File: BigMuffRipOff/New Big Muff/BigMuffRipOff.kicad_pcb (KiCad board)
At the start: 4 copper layers, 59.3 x 32 mm, 70 parts, among them J1 Conn_02x08_Odd_Even, Q1 BC549, Q2 BC549, Q3 BC549, Q4 BC549, U1 TPL0501-100DCNR, U10 LM2940IMP-9.0/NOPB, U2 TPL0501-100DCNR, U3 TPL0501-100DCNR, U4 TL071HIDBVR, U5 TL071HIDBVR, U6 ADP7118AUJZ-4.5-R7, U7 TL071HIDBVR, U8 TPL0501-100DCNR

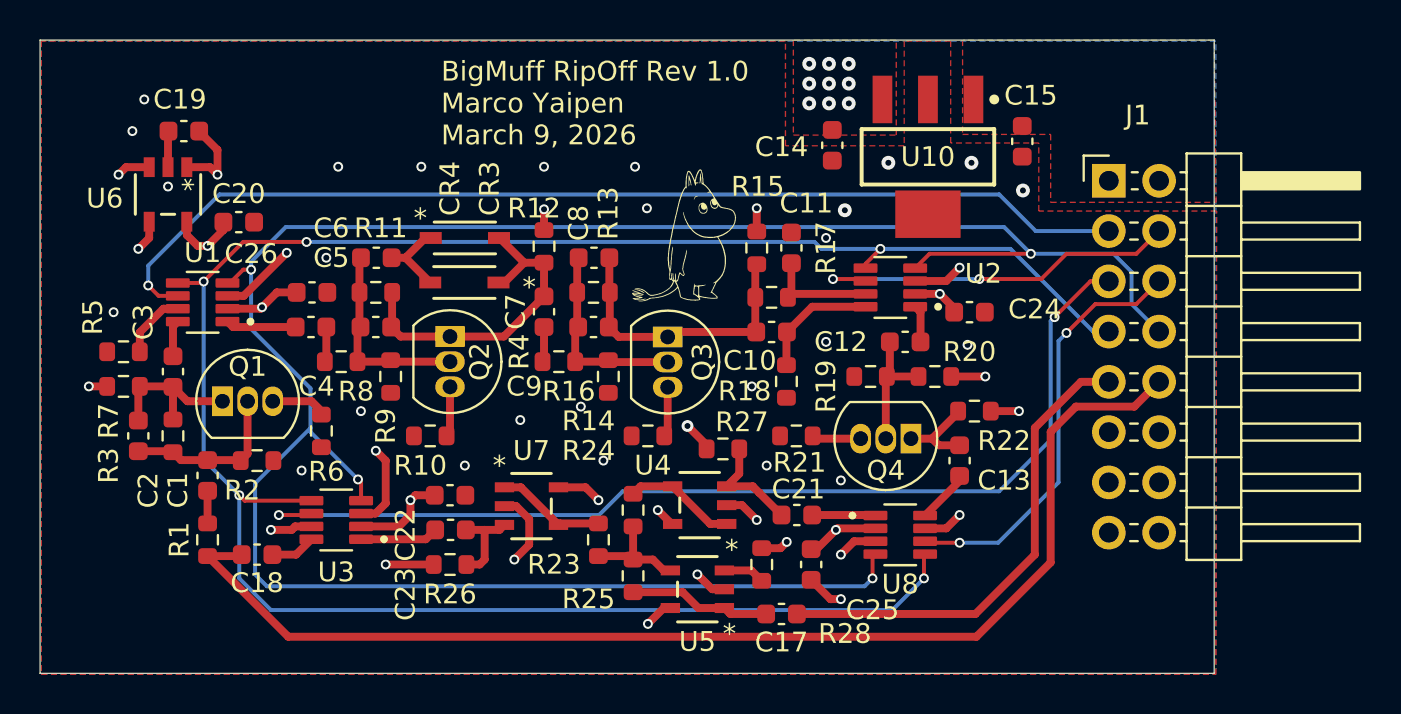
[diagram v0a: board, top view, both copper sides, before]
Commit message: big muff connector fixed i think?
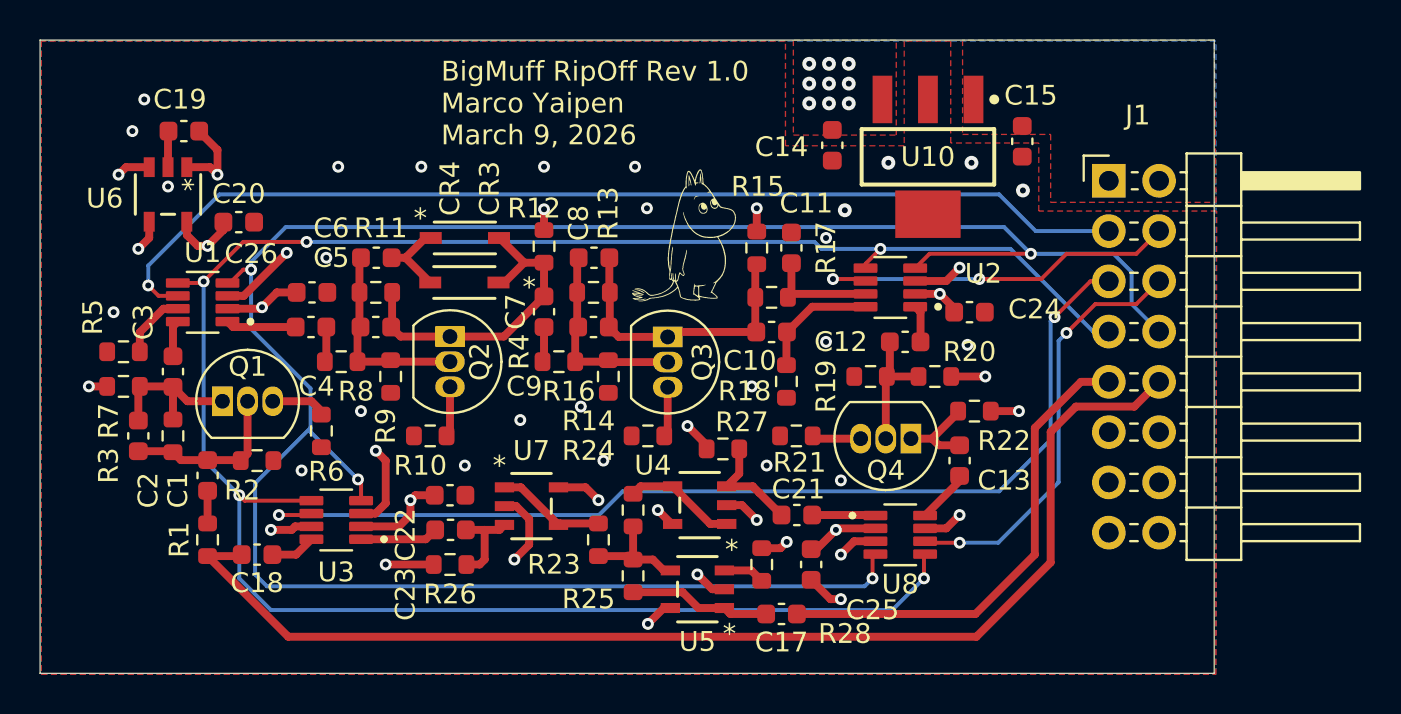
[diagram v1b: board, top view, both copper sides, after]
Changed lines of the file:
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@@
 	(via
 		(at 135.2 95.75)
-		(size 0.5)
+		(size 0.6)
 		(drill 0.3)
 		(layers "F.Cu" "B.Cu")
@@
 	(via
 		(at 152 92.25)
-		(size 0.5)
+		(size 0.6)
 		(drill 0.3)
 		(layers "F.Cu" "B.Cu")
@@
 	(via
 		(at 128.2 75.6)
-		(size 0.5)
+		(size 0.6)
 		(drill 0.3)
 		(layers "F.Cu" "B.Cu")
@@
 	(via
 		(at 160.25 92.5)
-		(size 0.5)
+		(size 0.6)
 		(drill 0.3)
 		(layers "F.Cu" "B.Cu")
@@
 	(via
 		(at 127.25 84.75)
-		(size 0.5)
+		(size 0.6)
 		(drill 0.3)
 		(layers "F.Cu" "B.Cu")
@@
 	(via
 		(at 163.25 86.25)
-		(size 0.5)
+		(size 0.6)
 		(drill 0.3)
 		(layers "F.Cu" "B.Cu")
@@
 	(via
 		(at 145 92.5)
-		(size 0.5)
+		(size 0.6)
 		(drill 0.3)
 		(layers "F.Cu" "B.Cu")
@@
 	(via
 		(at 159.75 95.25)
-		(size 0.5)
+		(size 0.6)
 		(drill 0.3)
 		(layers "F.Cu" "B.Cu")
@@
 	(via
 		(at 138 82)
-		(size 0.5)
+		(size 0.6)
 		(drill 0.3)
 		(layers "F.Cu" "B.Cu")
@@
 	(via
 		(at 136.75 92.75)
-		(size 0.5)
+		(size 0.6)
 		(drill 0.3)
 		(layers "F.Cu" "B.Cu")
@@
 	(via
 		(at 163.25 81)
-		(size 0.5)
+		(size 0.6)
 		(drill 0.3)
 		(layers "F.Cu" "B.Cu")
@@
 	(via
 		(at 154.2 79.5)
-		(size 0.5)
+		(size 0.6)
 		(drill 0.3)
 		(layers "F.Cu" "B.Cu")
@@
 	(via
 		(at 153.6 77.4)
-		(size 0.5)
+		(size 0.6)
 		(drill 0.3)
 		(layers "F.Cu" "B.Cu")
@@
 	(via
 		(at 142.8 77.4)
-		(size 0.5)
+		(size 0.6)
 		(drill 0.3)
 		(layers "F.Cu" "B.Cu")
@@
 	(via
 		(at 170 82.5)
-		(size 0.5)
+		(size 0.6)
 		(drill 0.3)
 		(layers "F.Cu" "B.Cu")
@@
 	(via
 		(at 149 77.4)
-		(size 0.5)
+		(size 0.6)
 		(drill 0.3)
 		(layers "F.Cu" "B.Cu")
@@
 	(via
 		(at 164 99.25)
-		(size 0.5)
+		(size 0.6)
 		(drill 0.3)
 		(layers "F.Cu" "B.Cu")
@@
 	(via
 		(at 164 97)
-		(size 0.5)
+		(size 0.6)
 		(drill 0.3)
 		(layers "F.Cu" "B.Cu")
@@
 	(via
 		(at 170 95)
-		(size 0.5)
+		(size 0.6)
 		(drill 0.3)
 		(layers "F.Cu" "B.Cu")
@@
 	(via
 		(at 147.8 90.2)
-		(size 0.5)
+		(size 0.6)
 		(drill 0.3)
 		(layers "F.Cu" "B.Cu")
@@
 	(via
 		(at 130 78.4)
-		(size 0.5)
+		(size 0.6)
 		(drill 0.3)
 		(layers "F.Cu" "B.Cu")
@@
 	(via
 		(at 139.75 89.75)
-		(size 0.5)
+		(size 0.6)
 		(drill 0.3)
 		(layers "F.Cu" "B.Cu")
@@
 	(via
 		(at 140.5 91.75)
-		(size 0.5)
+		(size 0.6)
 		(drill 0.3)
 		(layers "F.Cu" "B.Cu")
@@
 	(via
 		(at 156.75 98)
-		(size 0.5)
+		(size 0.6)
 		(drill 0.3)
 		(layers "F.Cu" "B.Cu")
@@
 	(via
 		(at 136 81.75)
-		(size 0.5)
+		(size 0.6)
 		(drill 0.3)
 		(layers "F.Cu" "B.Cu")
@@
 	(via
 		(at 147.5 97.25)
-		(size 0.5)
+		(size 0.6)
 		(drill 0.3)
 		(layers "F.Cu" "B.Cu")
@@
 	(via
 		(at 170.4 86.4)
-		(size 0.5)
+		(size 0.6)
 		(drill 0.3)
 		(layers "F.Cu" "B.Cu")
@@
 	(via
 		(at 150.860363 89.520726)
-		(size 0.5)
+		(size 0.6)
 		(drill 0.3)
 		(layers "F.Cu" "B.Cu")
@@
 	(via
 		(at 164 93.25)
-		(size 0.5)
+		(size 0.6)
 		(drill 0.3)
 		(layers "F.Cu" "B.Cu")
@@
 	(via
 		(at 128.8 74)
-		(size 0.5)
+		(size 0.6)
 		(drill 0.3)
 		(layers "F.Cu" "B.Cu")
@@
 	(via
 		(at 138.6 77.4)
-		(size 0.5)
+		(size 0.6)
 		(drill 0.3)
 		(layers "F.Cu" "B.Cu")
@@
 	(via
 		(at 159.5 88.5)
-		(size 0.5)
+		(size 0.6)
 		(drill 0.3)
 		(layers "F.Cu" "B.Cu")
@@
 	(via
 		(at 127.5 77.8)
-		(size 0.5)
+		(size 0.6)
 		(drill 0.3)
 		(layers "F.Cu" "B.Cu")
@@
 	(via
 		(at 132.5 77.8)
-		(size 0.5)
+		(size 0.6)
 		(drill 0.3)
 		(layers "F.Cu" "B.Cu")
@@
 	(via
 		(at 154.25 100.5)
-		(size 0.5)
+		(size 0.6)
 		(drill 0.3)
 		(layers "F.Cu" "B.Cu")
@@
 	(via
 		(at 126 88.5)
-		(size 0.5)
+		(size 0.6)
 		(drill 0.3)
 		(layers "F.Cu" "B.Cu")
@@
 	(via
 		(at 173 89.75)
-		(size 0.5)
+		(size 0.6)
 		(drill 0.3)
 		(layers "F.Cu" "B.Cu")
@@
 	(via
 		(at 149 79.55)
-		(size 0.5)
+		(size 0.6)
 		(drill 0.3)
 		(layers "F.Cu" "B.Cu")
@@
 	(via
 		(at 154.75 94.75)
-		(size 0.5)
+		(size 0.6)
 		(drill 0.3)
 		(layers "F.Cu" "B.Cu")
@@
 	(via
 		(at 159.75 79.5)
-		(size 0.5)
+		(size 0.6)
 		(drill 0.3)
 		(layers "F.Cu" "B.Cu")
@@
 	(via
 		(at 171.3 88)
-		(size 0.5)
+		(size 0.6)
 		(drill 0.3)
 		(layers "F.Cu" "B.Cu")
@@
 	(via
 		(at 151.75 94.25)
-		(size 0.5)
+		(size 0.6)
 		(drill 0.3)
 		(layers "F.Cu" "B.Cu")
@@
 	(via
 		(at 129 83.4)
-		(size 0.5)
+		(size 0.6)
 		(drill 0.3)
 		(layers "F.Cu" "B.Cu")
@@
 	(via
 		(at 135.6 95)
-		(size 0.5)
+		(size 0.6)
 		(drill 0.3)
 		(layers "F.Cu" "B.Cu")
@@
 	(via
 		(at 174.8 85)
-		(size 0.5)
+		(size 0.6)
 		(drill 0.3)
 		(layers "F.Cu" "B.Cu")
@@
 	(via
 		(at 131.8 83.2)
-		(size 0.5)
+		(size 0.6)
 		(drill 0.3)
 		(layers "F.Cu" "B.Cu")
@@
 	(via
 		(at 133.6 94)
-		(size 0.5)
+		(size 0.6)
 		(drill 0.3)
 		(layers "F.Cu" "B.Cu")
@@
 	(via
 		(at 166 81.551)
-		(size 0.5)
+		(size 0.6)
 		(drill 0.3)
 		(layers "F.Cu" "B.Cu")
@@
 	(via
 		(at 168.2 98.2)
-		(size 0.5)
+		(size 0.6)
 		(drill 0.3)
 		(layers "F.Cu" "B.Cu")
@@
 	(via
 		(at 137 81.2)
-		(size 0.5)
+		(size 0.6)
 		(drill 0.3)
 		(layers "F.Cu" "B.Cu")
@@
 	(via
 		(at 139.6 93.2)
-		(size 0.5)
+		(size 0.6)
 		(drill 0.3)
 		(layers "F.Cu" "B.Cu")
@@
 	(via
 		(at 134.2 82.6)
-		(size 0.5)
+		(size 0.6)
 		(drill 0.3)
 		(layers "F.Cu" "B.Cu")
@@
 	(via
 		(at 165.6 98.2)
-		(size 0.5)
+		(size 0.6)
 		(drill 0.3)
 		(layers "F.Cu" "B.Cu")
@@
 	(via
 		(at 173.6 81.8)
-		(size 0.5)
+		(size 0.6)
 		(drill 0.3)
 		(layers "F.Cu" "B.Cu")
@@
 	(via
 		(at 170 96.4)
-		(size 0.5)
+		(size 0.6)
 		(drill 0.3)
 		(layers "F.Cu" "B.Cu")
@@
 	(via
 		(at 175.4 85.8)
-		(size 0.5)
+		(size 0.6)
 		(drill 0.3)
 		(layers "F.Cu" "B.Cu")
@@
 	(via
 		(at 163.6 83.075)
-		(size 0.5)
+		(size 0.6)
 		(drill 0.3)
 		(layers "F.Cu" "B.Cu")
@@
 	(via
 		(at 171 83.075)
-		(size 0.5)
+		(size 0.6)
 		(drill 0.3)
 		(layers "F.Cu" "B.Cu")
@@
 	(via
 		(at 141 97.5)
-		(size 0.5)
+		(size 0.6)
 		(drill 0.3)
 		(layers "F.Cu" "B.Cu")
@@
 	(via
 		(at 132 81.4)
-		(size 0.5)
+		(size 0.6)
 		(drill 0.3)
 		(layers "F.Cu" "B.Cu")
@@
 	(via
 		(at 169 83.825)
-		(size 0.5)
+		(size 0.6)
 		(drill 0.3)
 		(layers "F.Cu" "B.Cu")
@@
 	(via
 		(at 142.25 94.25)
-		(size 0.5)
+		(size 0.6)
 		(drill 0.3)
 		(layers "F.Cu" "B.Cu")
@@
 	(via
 		(at 134.75 84.5)
-		(size 0.5)
+		(size 0.6)
 		(drill 0.3)
 		(layers "F.Cu" "B.Cu")
@@
 	(via
 		(at 163.75 95.75)
-		(size 0.5)
+		(size 0.6)
 		(drill 0.3)
 		(layers "F.Cu" "B.Cu")
@@
 	(via
 		(at 161.264827 96.358702)
-		(size 0.5)
+		(size 0.6)
 		(drill 0.3)
 		(layers "F.Cu" "B.Cu")
@@
 	(via
 		(at 128.5 81.55)
-		(size 0.5)
-		(drill 0.3)
-		(layers "F.Cu" "B.Cu")
+		(size 0.6)
+		(drill 0.3)
+		(layers "F.Cu" "B.Cu")
